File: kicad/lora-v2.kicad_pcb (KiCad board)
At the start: 4 copper layers, 47.5 x 43.5 mm, 55 parts, among them J1 USB_C_Receptacle_USB2.0_16P, SW1 bootsl, SW2 reset, U1 RP2040, U2 SX1262IMLTRT, U3 4259-63, U4 AP2112K-3.3TRG1, U5 W25Q16JVSS, Y1 32MHz, Y2 12MHz

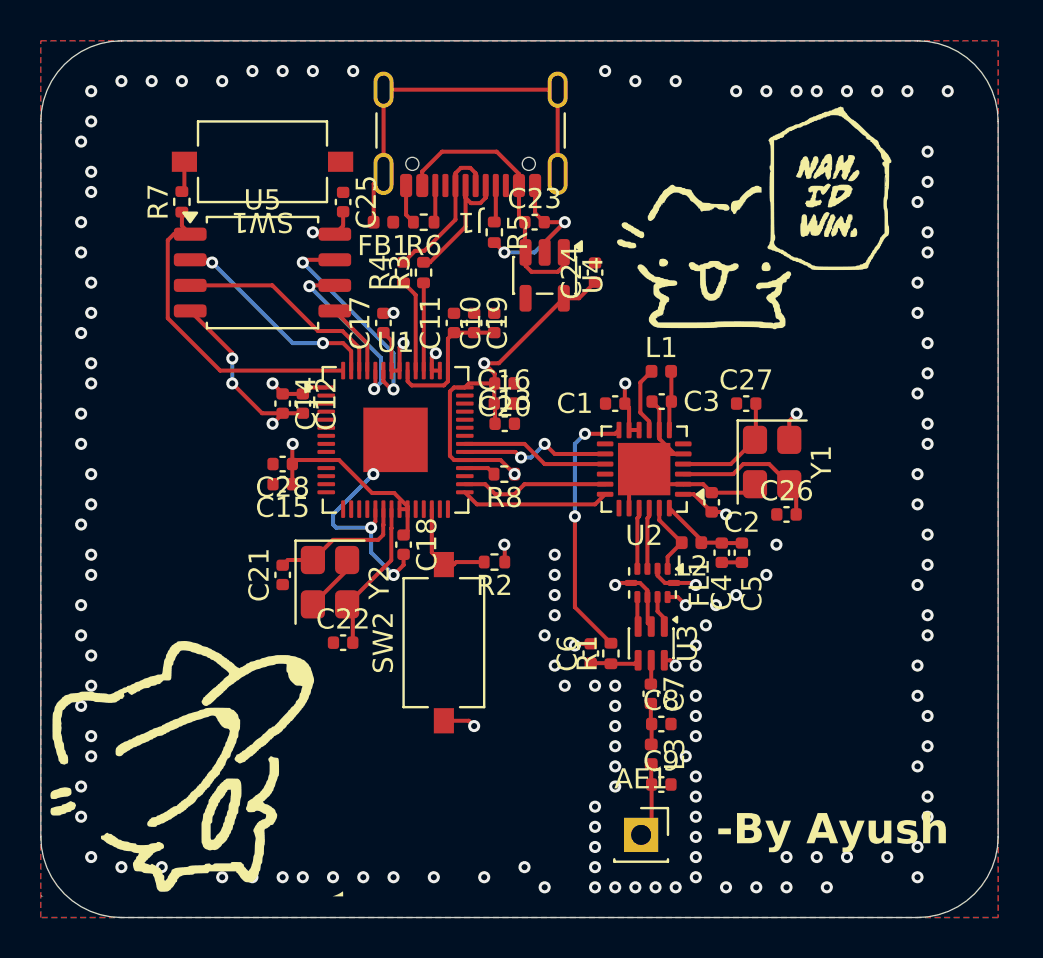
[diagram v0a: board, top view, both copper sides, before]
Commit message: added
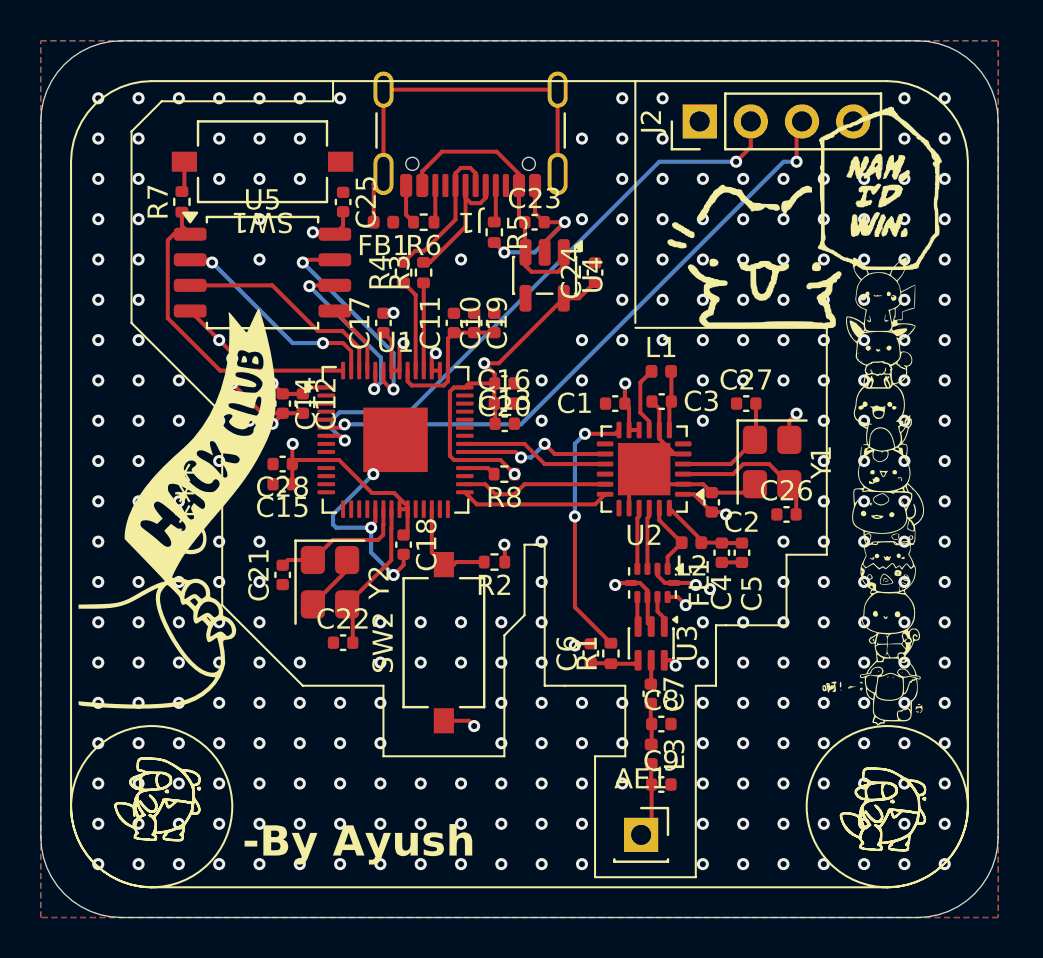
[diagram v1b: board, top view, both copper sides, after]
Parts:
- removed the G*** at (170.0, 100.5)
- added G*** (x2): LOGO, LOGO, F.Cu at (204.5, 103.0)
- added G***: LOGO, LOGO, B.Cu at (185.6, 82.4)
- added G***: LOGO, LOGO, B.Cu at (168.4, 102.2)
- added G*** (x2): LOGO, LOGO, F.Cu at (168.5, 102.5)
- added G***: LOGO, LOGO, F.Cu at (204.5, 87.0)
- added G***: LOGO, LOGO, F.Cu at (170.0, 88.2)
- added G***: LOGO, LOGO, B.Cu at (176.5, 81.8)
- added G***: LOGO, LOGO, B.Cu at (204.2, 103.4)
- added J2: Conn_01x04, Connector_PinHeader_2.54mm:PinHeader_1x04_P2.54mm_Vertical, F.Cu at (195.2, 69.0)
- moved G*** 21.2 mm to (198.0, 73.7)
- moved G*** 2.50 mm to (200.0, 74.0)
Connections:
- U1 pad 6: unconnected-(U1-GPIO4-Pad6) -> /SDA
- U1 pad 7: unconnected-(U1-GPIO5-Pad7) -> /SCL
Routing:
- net /SDA: track 0.00 -> 30.8 mm, vias 0 -> 2
- net /SCL: track 0.00 -> 30.0 mm, vias 0 -> 2
- net Earth: vias 152 -> 298
